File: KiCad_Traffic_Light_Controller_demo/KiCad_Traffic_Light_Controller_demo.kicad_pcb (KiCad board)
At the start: 2 copper layers, 64 parts, among them J1 Conn_02x08_Odd_Even, J2 Conn_02x08_Odd_Even, J3 Conn_02x05_Odd_Even, J4 +5V, SW1 RST, SW2 OVR, SW3 EN, U1 SM420561N, U2 SM420561N, U3 LM1117DT-3.3

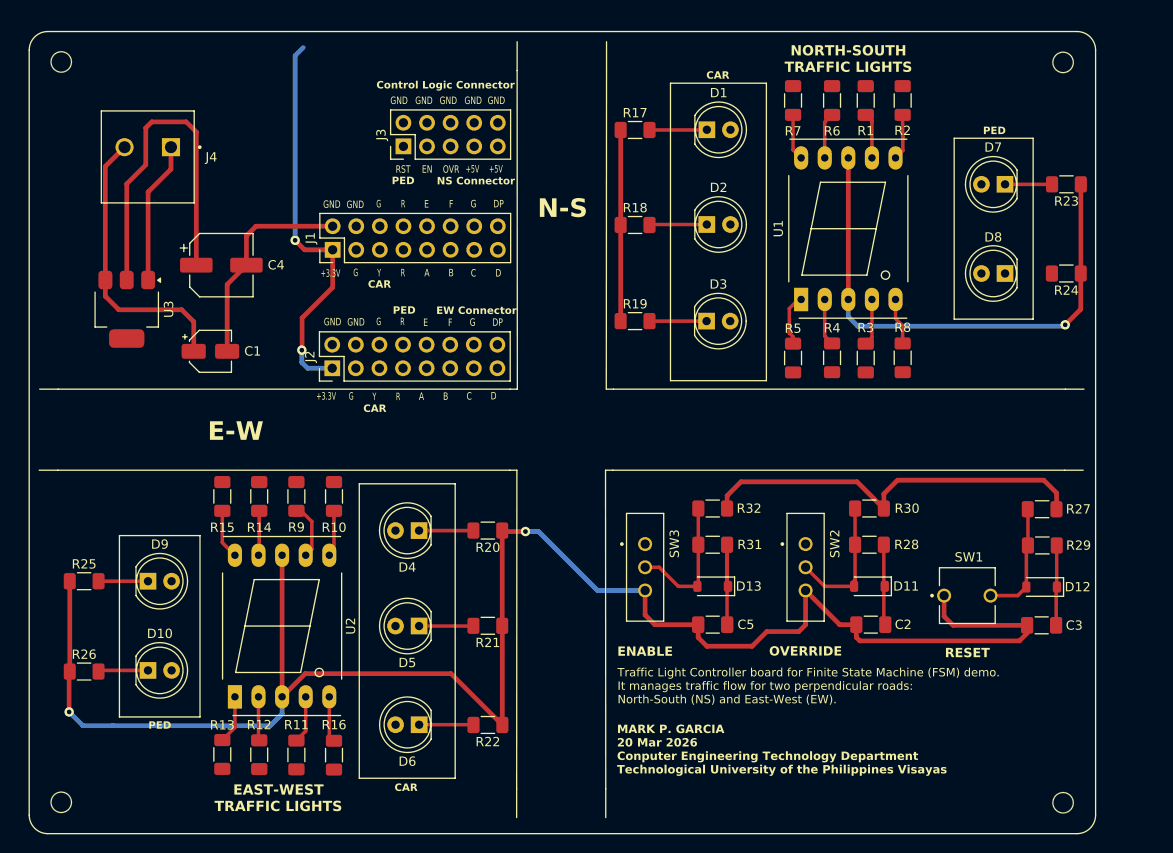
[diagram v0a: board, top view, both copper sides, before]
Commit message: Updated
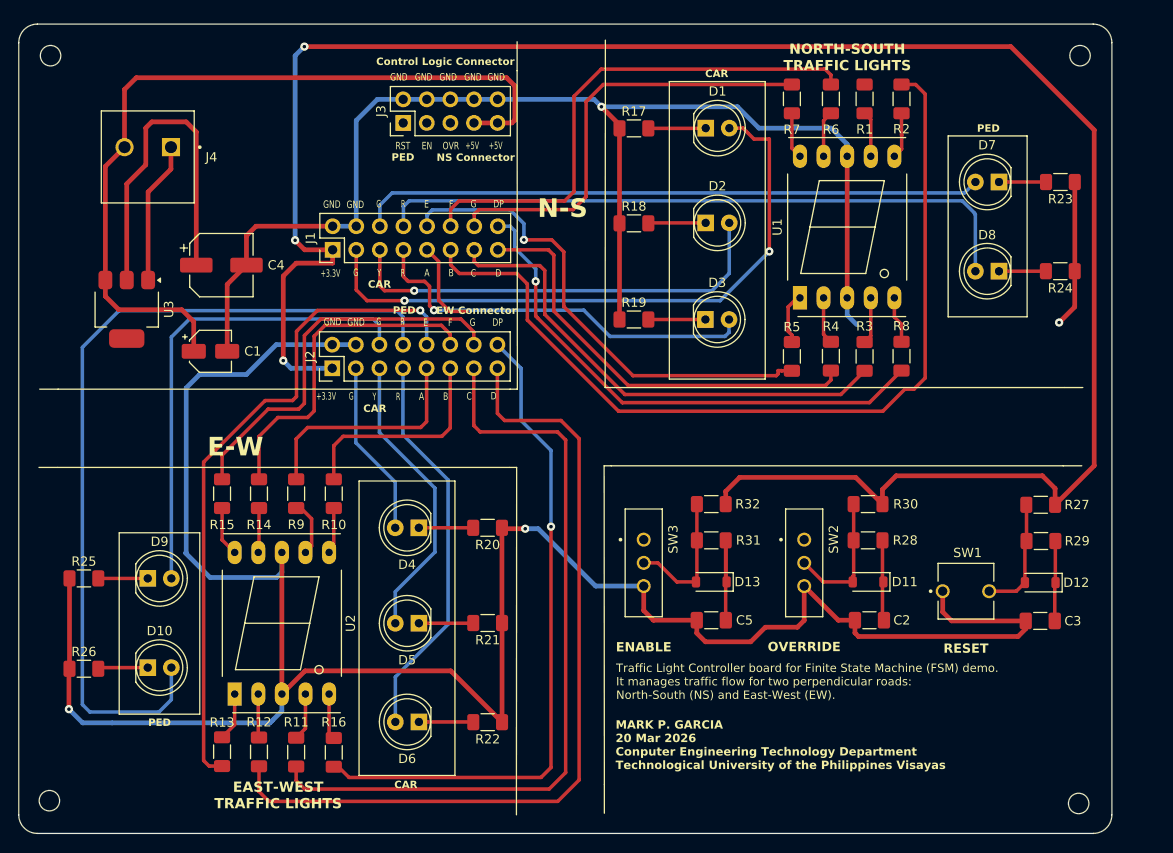
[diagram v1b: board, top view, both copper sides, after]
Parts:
- moved J3 2.53 mm to (139.1, 49.1)
- moved H3 1.96 mm to (212.0, 41.9)
- moved H2 1.68 mm to (211.8, 122.4)
- moved H4 1.33 mm to (101.2, 41.9)
- moved H1 1.29 mm to (101.0, 122.1)
- moved D7 0.70 mm to (203.2, 55.5)
- moved D8 0.70 mm to (203.2, 65.1)
- moved R24 0.70 mm to (209.8, 65.1)
- moved R23 0.70 mm to (209.9, 55.5)
- moved C3 0.50 mm to (207.7, 102.7)
- moved D12 0.50 mm to (207.7, 98.6)
- moved R27 0.50 mm to (207.7, 90.2)
- moved R28 0.50 mm to (189.2, 94.0)
- moved R31 0.50 mm to (172.3, 94.0)
- moved SW2 0.50 mm to (182.3, 96.5)
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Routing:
- net /+3.3V: track 123.5 -> 259.5 mm, vias 2 -> 3
- net GND: track 303.3 -> 406.9 mm, vias 3 -> 4
- net /NS_HEX_B: track 0.00 -> 96.5 mm
- net /EWP_RED: track 0.00 -> 91.8 mm
- net /EW_HEX_D: track 0.00 -> 90.1 mm
- net /EW_HEX_C: track 0.00 -> 84.1 mm
- net /EW_HEX_E: track 0.00 -> 72.5 mm, vias 0 -> 1
- net /EW_HEX_DP: track 0.00 -> 72.2 mm, vias 0 -> 1
- net /NSP_RED: track 0.00 -> 70.7 mm
- net /NSC_GRN: track 0.00 -> 68.3 mm, vias 0 -> 2
- net /NSP_GRN: track 0.00 -> 67.4 mm
- net /+5V: track 30.7 -> 88.0 mm
- net /NS_HEX_DP: track 0.00 -> 56.8 mm, vias 0 -> 1
- net /NS_HEX_F: track 0.00 -> 56.3 mm
- net /NS_HEX_C: track 0.00 -> 53.0 mm
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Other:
- board outline added: 117.7 x 87.1 mm

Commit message: Updated
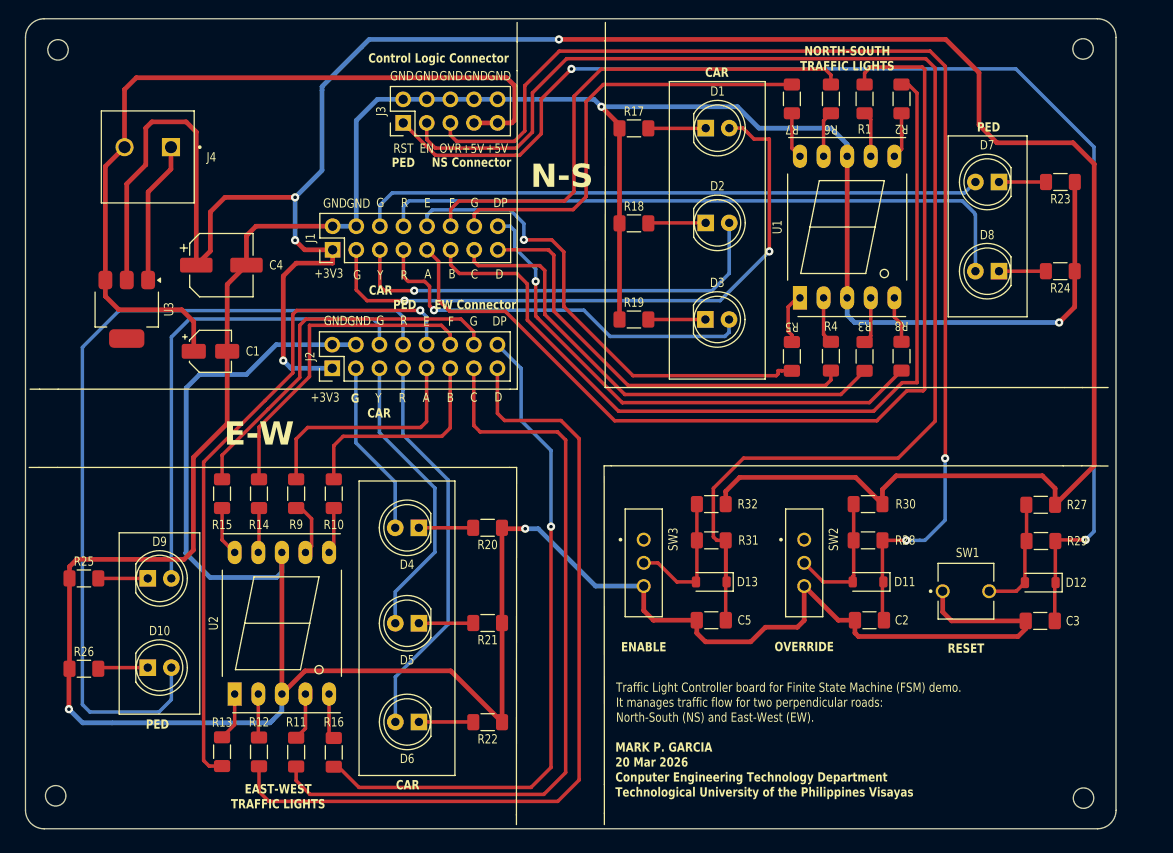
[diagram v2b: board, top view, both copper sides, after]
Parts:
- D4: value EWC_GRN -> GREEN
- D5: value EWC_YLW -> YELLOW
- D6: value EWC_RED -> RED
- moved H4 1.02 mm to (102.0, 41.2)
- moved H1 0.86 mm to (101.7, 121.5)
- moved H3 0.79 mm to (212.3, 41.1)
- moved H2 0.78 mm to (212.3, 121.8)
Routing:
- net /EN: track 13.1 -> 148.5 mm
- net /RST: track 8.65 -> 140.0 mm, vias 0 -> 2
- net /OVR: track 8.67 -> 127.6 mm, vias 0 -> 2
- net /NS_HEX_A: track 9.49 -> 107.6 mm
- net GND: track 406.9 -> 466.8 mm
- net /+3.3V: track 259.5 -> 273.8 mm, vias 3 -> 4
- net /NS_HEX_B: track 96.5 -> 95.1 mm
- net /EW_HEX_G: track 42.0 -> 41.0 mm
- net /EW_HEX_F: track 36.4 -> 35.5 mm
- net /EW_HEX_DP: track 72.2 -> 73.1 mm
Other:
- board size 117.7 x 87.1 mm -> 117.4 x 87.2 mm
- board text added: "+3V3"
- board text removed: "+3.3V"
